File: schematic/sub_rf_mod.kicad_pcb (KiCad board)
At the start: 2 copper layers, 69.1 x 50 mm, 39 parts, among them J4B1 Conn_01x08

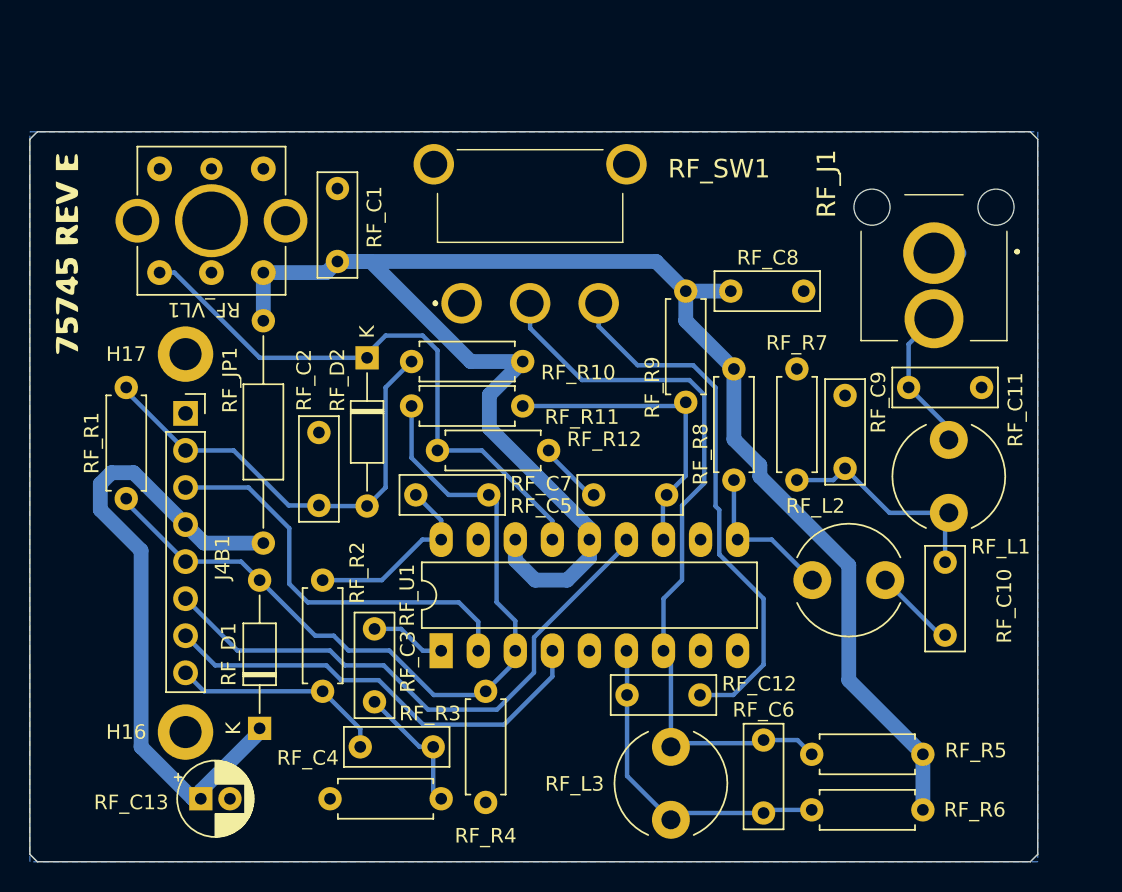
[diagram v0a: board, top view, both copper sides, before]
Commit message: cleanup for release of version 1
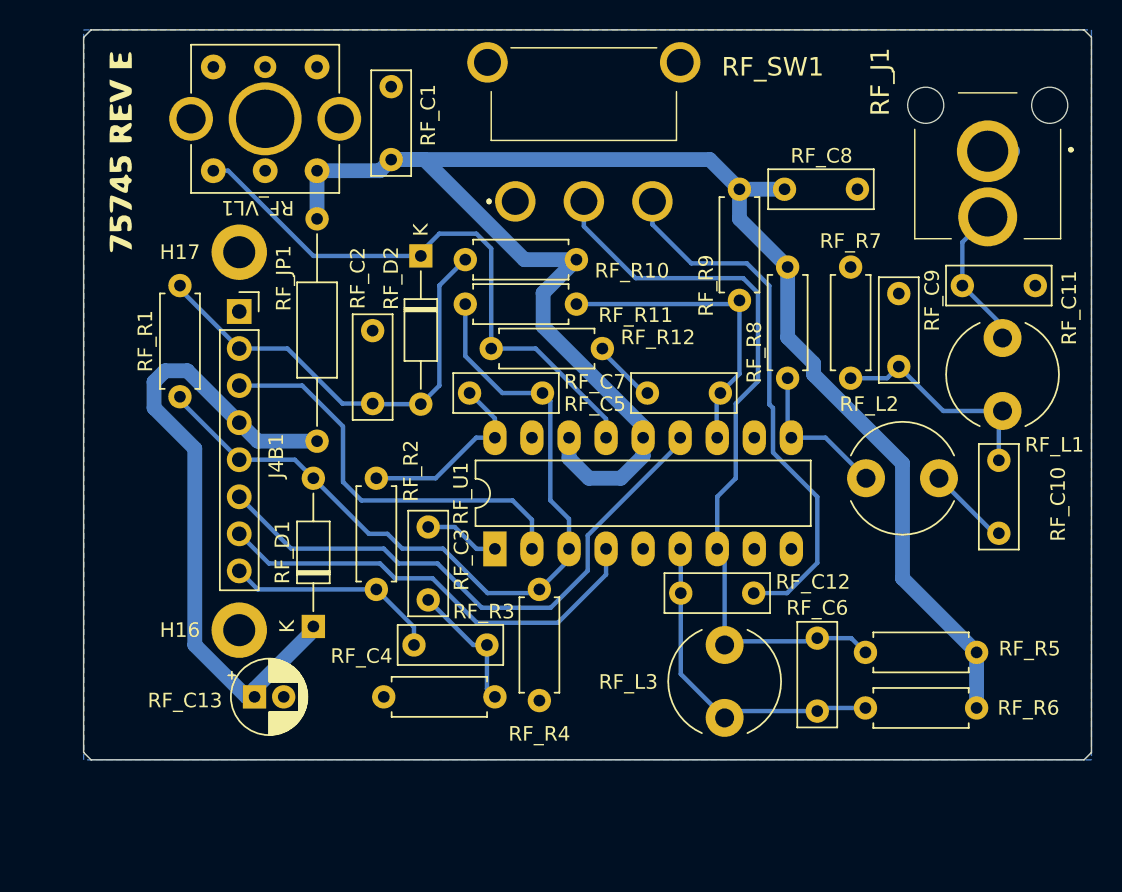
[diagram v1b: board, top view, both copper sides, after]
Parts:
- moved RF_C3 7.90 mm to (134.7, 91.1)
- moved RF_L3 7.90 mm to (155.1, 99.2)
- moved RF_R10 7.90 mm to (144.9, 72.8)
- moved RF_R3 7.90 mm to (131.7, 102.7)
- moved RF_C8 7.90 mm to (159.2, 67.9)
- moved RF_R5 7.90 mm to (172.3, 99.7)
- moved RF_R9 7.90 mm to (156.1, 67.9)
- moved H16 7.90 mm to (121.8, 98.2)
- moved H17 7.90 mm to (121.8, 72.3)
- moved J4B1 7.90 mm to (121.8, 76.3)
- moved RF_C2 7.90 mm to (130.9, 77.6)
- moved RF_D1 7.90 mm to (126.9, 97.9)
- moved RF_R2 7.90 mm to (131.2, 87.8)
- moved S5 7.90 mm to (113.7, 65.4)
- moved RF_C1 7.90 mm to (132.2, 65.9)
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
